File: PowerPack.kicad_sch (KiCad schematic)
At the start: 75 parts, among them CN1 XT30PW-M, Q1 WSD3066DN33, U1 IP2368_BZ_VGLIP_C5203723, U2 ME6203A50PG

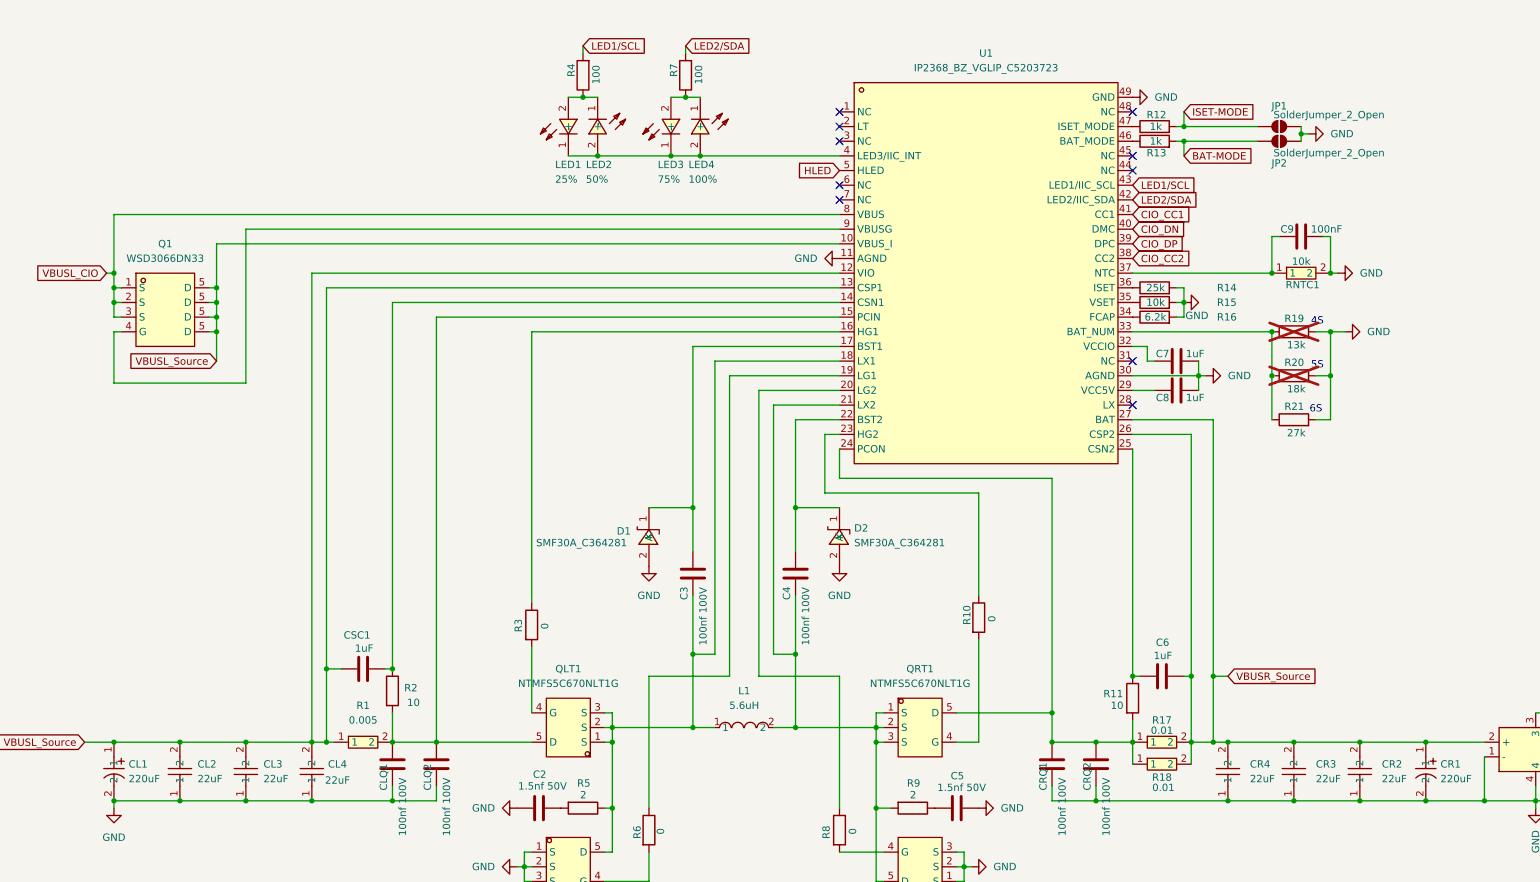
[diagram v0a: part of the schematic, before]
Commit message: route pcb
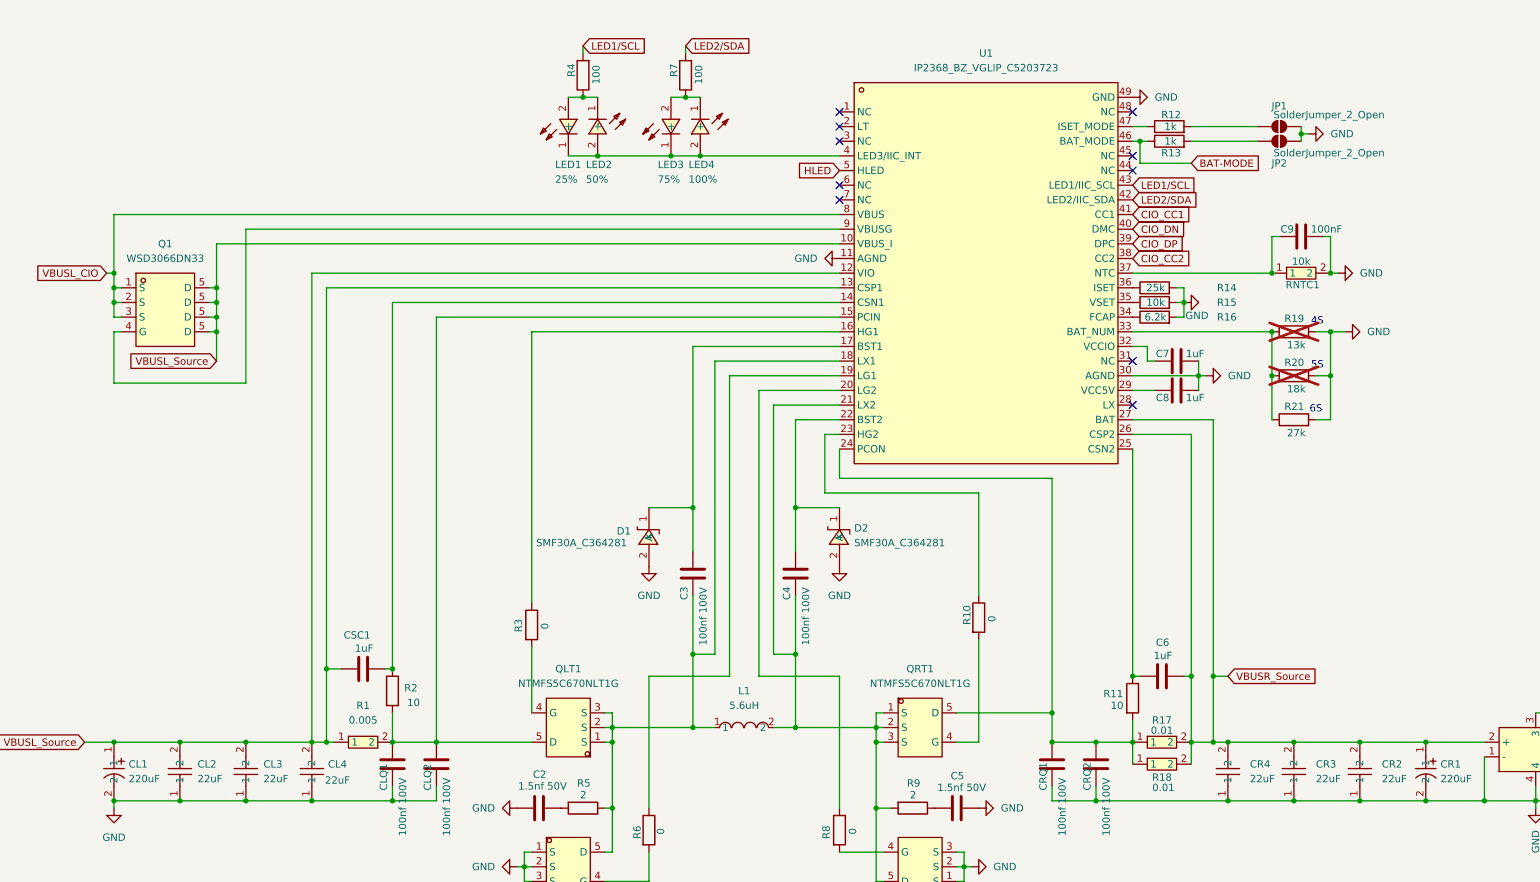
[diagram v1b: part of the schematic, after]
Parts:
- C12, C13: value 100nf -> 100nf
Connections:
- net BAT-MODE: now also R13.1, U1.46 (BAT_MODE); no longer JP2.1 (A), R13.2
- net ISET-MODE: no longer names the net of JP1.1 (A), R12.2
- new net: JP2.1 (A), R13.2
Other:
- moved on the sheet: R12, R13
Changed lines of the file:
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@@
 (kicad_sch
-	(version 20231120)
+	(version 20250114)
 	(generator "eeschema")
-	(generator_version "8.0")
+	(generator_version "9.0")
 	(paper "A3")
 	(title_block
 		(title "PowerPack")
 	)
+	(text "5S"
+		(exclude_from_sim no)
+		(at 249.174 177.292 0)
+		(effects
+			(font
+				(size 1.27 1.27)
+			)
+		)
+	)
+	(text "6S"
+		(exclude_from_sim no)
+		(at 248.92 184.912 0)
+		(effects
+			(font
+				(size 1.27 1.27)
+			)
+		)
+	)
+	(text "4S"
+		(exclude_from_sim no)
+		(at 249.174 169.672 0)
+		(effects
+			(font
+				(size 1.27 1.27)
+			)
+		)
+	)
 	(junction
 		(at 40.64 242.57)
@@
 	)
 	(junction
-		(at 226.06 138.43)
-		(diameter 0)
-		(color 0 0 0 0)
-	)
-	(junction
 		(at 332.74 46.99)
 		(diameter 0)
@@
 	)
 	(junction
-		(at 226.06 135.89)
-		(diameter 0)
-		(color 0 0 0 0)
-	)
-	(junction
 		(at 88.9 252.73)
 		(diameter 0)
@@
 	)
 	(junction
+		(at 218.44 138.43)
+		(diameter 0)
+		(color 0 0 0 0)
+	)
+	(junction
 		(at 88.9 229.87)
 		(diameter 0)
@@
 	(wire
 		(pts
+			(xy 227.33 135.89) (xy 238.76 135.89)
+		)
+		(stroke
+			(width 0)
+			(type default)
+		)
+	)
+	(wire
+		(pts
 			(xy 113.03 266.7) (xy 111.76 266.7)
 		)
@@
 	(wire
 		(pts
+			(xy 218.44 138.43) (xy 217.17 138.43)
+		)
+		(stroke
+			(width 0)
+			(type default)
+		)
+	)
+	(wire
+		(pts
 			(xy 393.7 25.4) (xy 393.7 35.56)
 		)
@@
 	(wire
 		(pts
-			(xy 226.06 138.43) (xy 224.79 138.43)
-		)
-		(stroke
-			(width 0)
-			(type default)
-		)
-	)
-	(wire
-		(pts
-			(xy 226.06 135.89) (xy 224.79 135.89)
-		)
-		(stroke
-			(width 0)
-			(type default)
-		)
-	)
-	(wire
-		(pts
 			(xy 166.37 231.14) (xy 166.37 254)
 		)
@@
 	(wire
 		(pts
-			(xy 238.76 135.89) (xy 226.06 135.89)
-		)
-		(stroke
-			(width 0)
-			(type default)
-		)
-	)
-	(wire
-		(pts
 			(xy 337.82 46.99) (xy 339.09 46.99)
 		)
@@
 	(wire
 		(pts
-			(xy 226.06 138.43) (xy 226.06 140.97)
-		)
-		(stroke
-			(width 0)
-			(type default)
-		)
-	)
-	(wire
-		(pts
 			(xy 40.64 161.29) (xy 40.64 163.83)
 		)
@@
 	(wire
 		(pts
+			(xy 218.44 142.24) (xy 218.44 138.43)
+		)
+		(stroke
+			(width 0)
+			(type default)
+		)
+	)
+	(wire
+		(pts
 			(xy 228.6 179.07) (xy 228.6 181.61)
 		)
@@
 	(wire
 		(pts
+			(xy 219.71 138.43) (xy 218.44 138.43)
+		)
+		(stroke
+			(width 0)
+			(type default)
+		)
+	)
+	(wire
+		(pts
 			(xy 52.07 242.57) (xy 63.5 242.57)
 		)
@@
 	(wire
 		(pts
+			(xy 227.33 142.24) (xy 218.44 142.24)
+		)
+		(stroke
+			(width 0)
+			(type default)
+		)
+	)
+	(wire
+		(pts
 			(xy 58.42 171.45) (xy 58.42 176.53)
 		)
@@
 	(wire
 		(pts
-			(xy 226.06 133.35) (xy 226.06 135.89)
-		)
-		(stroke
-			(width 0)
-			(type default)
-		)
-	)
-	(wire
-		(pts
 			(xy 248.92 171.45) (xy 251.46 171.45)
 		)
@@
 	(wire
 		(pts
+			(xy 219.71 135.89) (xy 217.17 135.89)
+		)
+		(stroke
+			(width 0)
+			(type default)
+		)
+	)
+	(wire
+		(pts
 			(xy 175.26 254) (xy 172.72 254)
 		)
@@
 	(wire
 		(pts
-			(xy 238.76 138.43) (xy 226.06 138.43)
+			(xy 227.33 138.43) (xy 238.76 138.43)
 		)
 		(stroke
@@
 		)
 	)
-	(text "5S"
-		(exclude_from_sim no)
-		(at 249.174 177.292 0)
-		(effects
-			(font
-				(size 1.27 1.27)
-			)
-		)
-	)
-	(text "6S"
-		(exclude_from_sim no)
-		(at 248.92 184.912 0)
-		(effects
-			(font
-				(size 1.27 1.27)
-			)
-		)
-	)
-	(text "4S"
-		(exclude_from_sim no)
-		(at 249.174 169.672 0)
-		(effects
-			(font
-				(size 1.27 1.27)
-			)
-		)
-	)
 	(global_label "HLED"
 		(shape input)
@@
 	(global_label "BAT-MODE"
 		(shape input)
-		(at 226.06 140.97 0)
+		(at 227.33 142.24 0)
 		(fields_autoplaced yes)
 		(effects
@@
 		)
 		(property "Intersheetrefs" "${INTERSHEET_REFS}"
-			(at 239.1447 140.97 0)
+			(at 240.4147 142.24 0)
 			(effects
 				(font
@@
 		)
 	)
-	(global_label "ISET-MODE"
-		(shape input)
-		(at 226.06 133.35 0)
-		(fields_autoplaced yes)
-		(effects
-			(font
-				(size 1.27 1.27)
-			)
-			(justify left)
-		)
-		(property "Intersheetrefs" "${INTERSHEET_REFS}"
-			(at 239.7494 133.35 0)
-			(effects
-				(font
-					(size 1.27 1.27)
-				)
-				(justify left)
-				(hide yes)
-			)
-		)
-	)
 	(global_label "VBUSL_CIO"
 		(shape input)
@@
 	(symbol
 		(lib_id "Device:R")
-		(at 220.98 135.89 90)
+		(at 223.52 135.89 90)
 		(unit 1)
 		(exclude_from_sim no)
@@
 		(dnp no)
 		(property "Reference" "R12"
-			(at 223.012 133.858 90)
+			(at 225.552 133.858 90)
 			(effects
 				(font
@@
 		)
 		(property "Value" "1k"
-			(at 222.25 135.89 90)
+			(at 224.79 135.89 90)
 			(effects
 				(font
@@
 		)
 		(property "Footprint" "Resistor_SMD:R_0402_1005Metric_Pad0.72x0.64mm_HandSolder"
-			(at 220.98 137.668 90)
+			(at 223.52 137.668 90)
 			(effects
 				(font
@@
 		)
 		(property "Datasheet" "~"
-			(at 220.98 135.89 0)
+			(at 223.52 135.89 0)
 			(effects
 				(font
@@
 		)
 		(property "Description" "Resistor"
-			(at 220.98 135.89 0)
+			(at 223.52 135.89 0)
 			(effects
 				(font
@@
 	(symbol
 		(lib_id "Device:R")
-		(at 220.98 138.43 90)
+		(at 223.52 138.43 90)
 		(unit 1)
 		(exclude_from_sim no)
@@
 		(dnp no)
 		(property "Reference" "R13"
-			(at 223.012 140.462 90)
+			(at 225.552 140.462 90)
 			(effects
 				(font
@@
 		)
 		(property "Value" "1k"
-			(at 222.25 138.43 90)
+			(at 224.79 138.43 90)
 			(effects
 				(font
@@
 		)
 		(property "Footprint" "Resistor_SMD:R_0402_1005Metric_Pad0.72x0.64mm_HandSolder"
-			(at 220.98 140.208 90)
+			(at 223.52 140.208 90)
 			(effects
 				(font
@@
 		)
 		(property "Datasheet" "~"
-			(at 220.98 138.43 0)
+			(at 223.52 138.43 0)
 			(effects
 				(font
@@
 		)
 		(property "Description" "Resistor"
-			(at 220.98 138.43 0)
+			(at 223.52 138.43 0)
 			(effects
 				(font
@@
 			)
 		)
-		(property "Value" "100nf "
+		(property "Value" "100nf"
 			(at 335.28 55.372 0)
 			(effects
@@
 			)
 		)
-		(property "Value" "100nf "
+		(property "Value" "100nf"
 			(at 375.92 57.912 0)
 			(effects
@@
 		)
 	)
+	(embedded_fonts no)
 )
